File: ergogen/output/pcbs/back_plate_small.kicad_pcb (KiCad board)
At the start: 2 copper layers, 127.5 x 91.9 mm, 6 parts

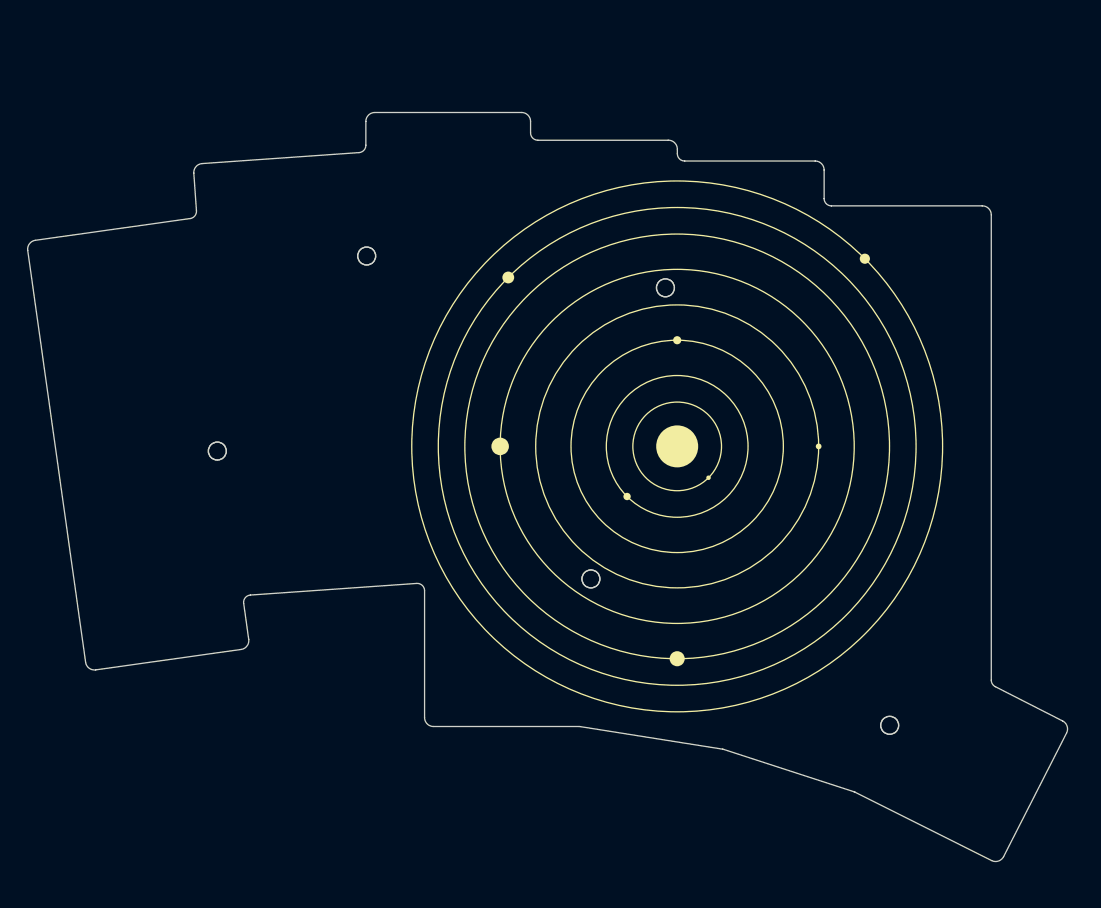
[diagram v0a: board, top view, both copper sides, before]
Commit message: new shape
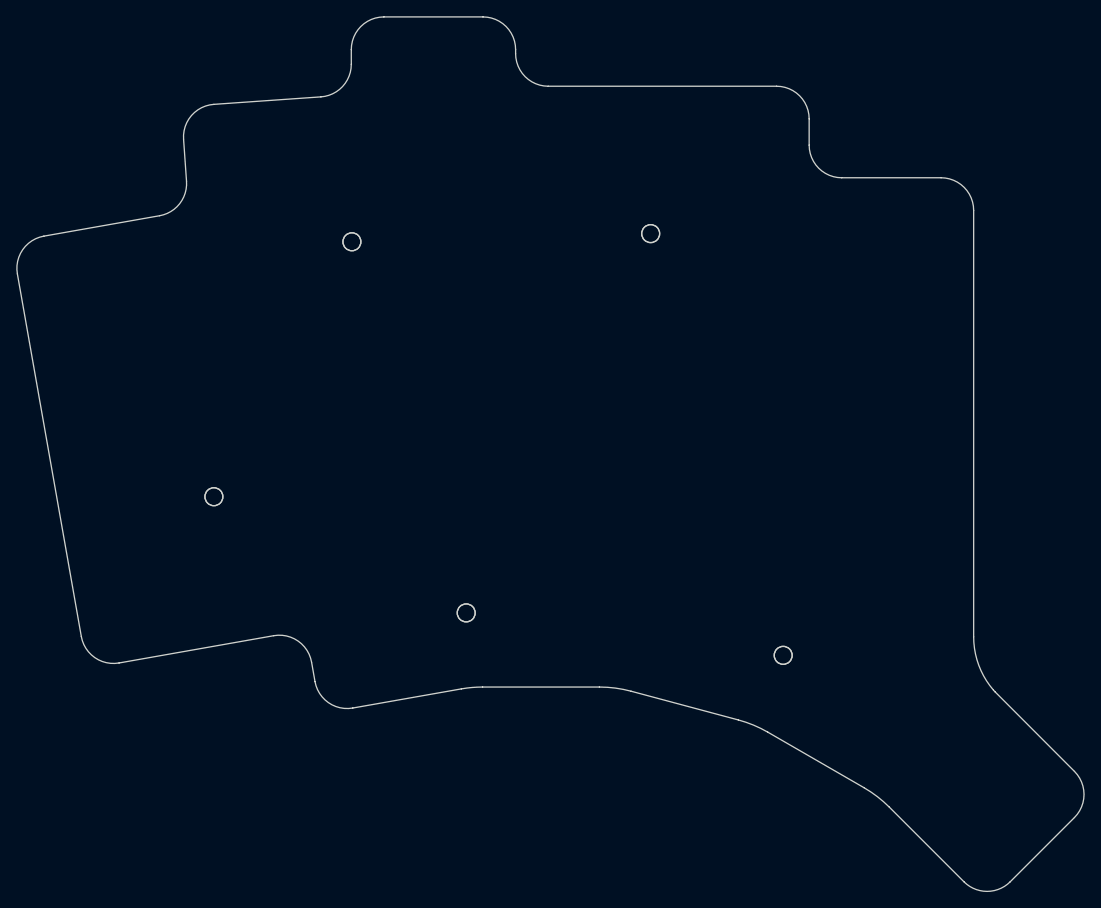
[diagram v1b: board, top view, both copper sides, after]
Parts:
- removed ?: , solar_system
- moved MH4 15.9 mm to (104.5, 92.8), turned to 10 degrees
- moved MH3 15.6 mm to (143.4, 98.1), turned to -15 degrees
- moved MH2 6.89 mm to (127.1, 46.3)
- moved MH5 5.62 mm to (73.6, 78.6)
- moved MH1 2.52 mm to (90.5, 47.3)
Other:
- board size 127.5 x 91.9 mm -> 130.9 x 107.2 mm
